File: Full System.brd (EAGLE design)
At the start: 47.5 x 21.5 mm, 46 parts, among them CN2 JSTPH, IC1 MEGA328-A, IC2 L4931D, Q1-M 8MHz, 22pF, U2 MCP73831T-2ACI/OT, U3 FTS31XS-U

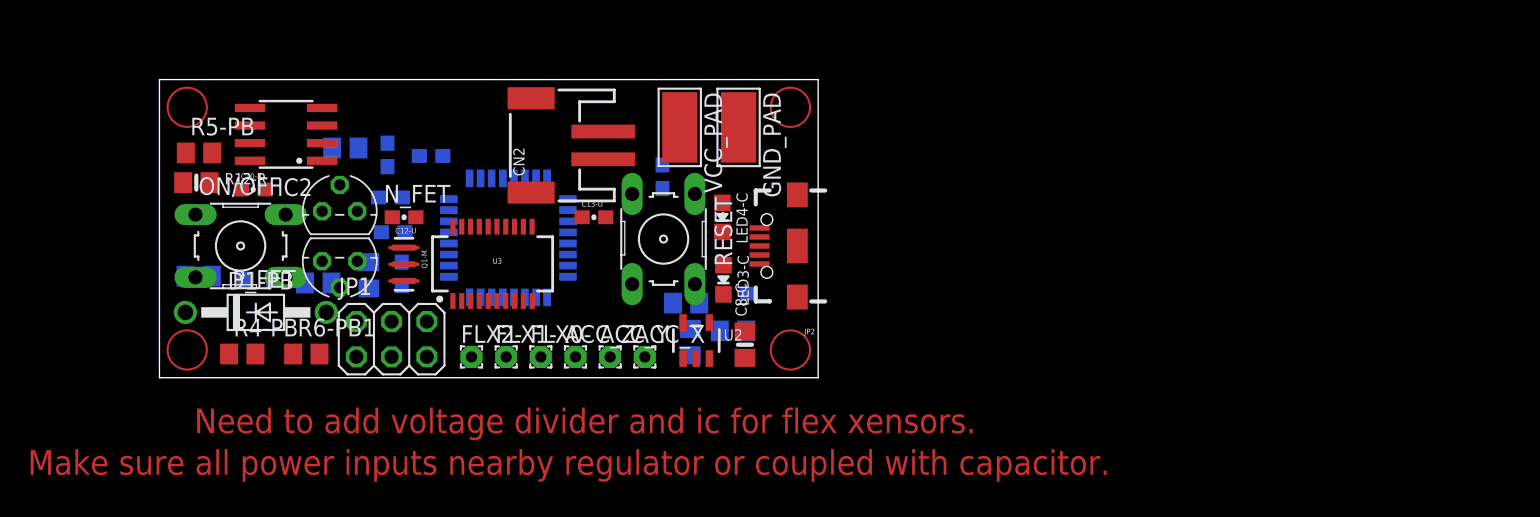
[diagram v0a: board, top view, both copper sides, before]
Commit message: Add files via upload
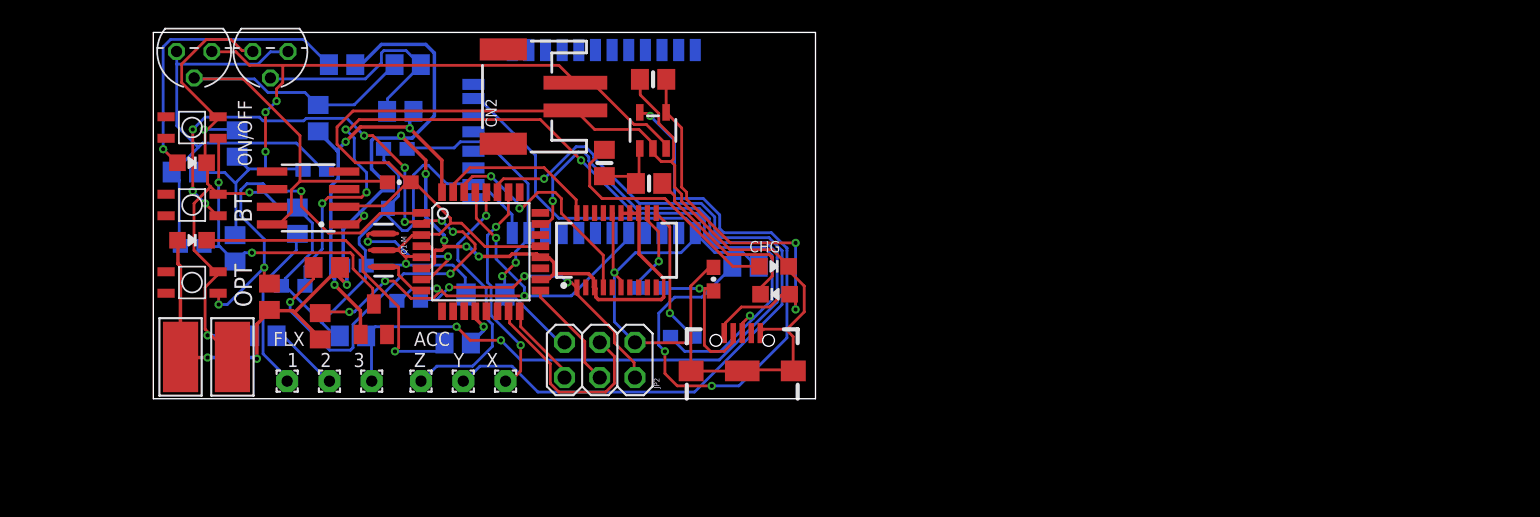
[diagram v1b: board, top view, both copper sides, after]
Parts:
- removed LED4-C: GREEN, microbuilder:CHIPLED_0805_NOOUTLINE
- removed ON/OFF, RESET: (no value), switch-omron:B3F-10XX
- removed R6-PB1: 10k, rcl:R0805
- added C1: 0.1uF, SparkFun:0603-CAP
- added C2: 10uF, SparkFun:EIA3216
- added CHG: GREEN, microbuilder:CHIPLED_0805_NOOUTLINE
- added LED2-M: Blue, microbuilder:CHIPLED_0805_NOOUTLINE
- added R1-M, R1-M1, R1-M2, R1-M3, R2-M, R2-M1, R3-M: 10k, rcl:R0805
- added S1: Power, Spark:TACTILE_SWITCH_SMD
- added S2: Option, Spark:TACTILE_SWITCH_SMD
- added S3: BT_C, Spark:TACTILE_SWITCH_SMD
- added U1: BLUETOOTH-RN41", SparkFun-RF:RN41
- D1-PB: value 1N4004 -> (none); device diode:DO41-10 -> semicon-smd-ipc:SOT23
- moved GND_PAD 40.1 mm to (9.26, 2.00)
- moved VCC_PAD 39.6 mm to (5.52, 2.00), turned to 0 degrees
- moved C14-U 27.5 mm to (18.1, 8.59), turned to 180 degrees
- moved C8-C 20.3 mm to (39.6, 22.0), turned to 180 degrees
- moved R13-U 18.5 mm to (39.5, 6.97)
- moved P_FET 18.4 mm to (6.50, 24.0)
- moved R4-PB 17.9 mm to (15.4, 19.2), flipped to the bottom, turned to 270 degrees
- moved U2 15.5 mm to (39.6, 18.3)
- moved R9-C 15.2 mm to (36.1, 16.0), flipped to the top, turned to 270 degrees
- moved JP1 15.1 mm to (35.7, 1.78)
- moved R5-PB 14.8 mm to (21.4, 19.7), flipped to the bottom, turned to 180 degrees
- moved C7-PB 14.5 mm to (6.36, 10.0)
- moved R12-R 13.5 mm to (17.2, 23.1), flipped to the bottom
- moved C9-C 13.4 mm to (9.60, 17.4), turned to 90 degrees
- moved FLX2- 13.4 mm to (13.2, 0.25)
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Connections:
- removed net N$13: IC1.12
- new net FLX1: FLX1-.1, R1-M2.1
- new net LED1: IC1.12, R2-M1.1
- new net N$10: LED2-M.C, R2-M1.2
- new net N$6: IC1.2, R3-M.1, S3.1
- new net PIO10: U1.33
- new net PIO11: U1.34
- new net PIO2: U1.19
- new net PIO3: U1.20
- new net PIO4: U1.22
- new net PIO5: U1.21
- new net PIO6: U1.3
- new net PIO7: U1.4
- new net RESET: C2-M.1, IC1.29, R1-M.2, U1.5
- new net SPICLK: U1.6
- new net SPICSB: U1.23
- new net SPIMISO: U1.24
- new net SPIMOSI: U1.2
- new net UARTCTS: U1.16
- new net UARTRTS: U1.15
- new net UARTRX: U1.13
- new net UARTTX: U1.14
- net 3.3V: now also LED2-M.A, R1-M.1, R2-M.2, R3-M.2; no longer R6-PB1.1
- net ACC_X: now also ACC_X.1
- net ACC_Y: now also ACC_Y.1
- net ACC_Z: now also ACC_Z.1
- net FLX0: now also FLX0-.1, R1-M1.1
- net GND: now also C1.2, C2.C, CHG.C, R1-M1.2, R1-M2.2, R1-M3.2, S1.2, S2.3, S3.3, U1.1, U1.12, U1.28, U1.29; no longer LED4-C.C, ON/OFF.3, ON/OFF.4, RESET.3, RESET.4
- net N$14: now also FLX2-.1, R1-M3.1; no longer IC1.13
- net N$19: now also CHG.A; no longer LED4-C.A
- net N$2: now also IC1.1, R2-M.1, S2.1; no longer C2-M.1, IC1.29, R6-PB1.2, RESET.1, RESET.2
- net N$5: now also D1-PB.3, S1.4; no longer D1-PB.C, ON/OFF.1, ON/OFF.2
- net POWER_OFF: now also D1-PB.1; no longer D1-PB.A
- net VCC: now also C1.1, C2.A, U1.11
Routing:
- net GND: track 0.00 -> 255.9 mm, vias 0 -> 5
- net 3.3V: track 0.00 -> 101.2 mm, vias 0 -> 9
- net N$12: track 0.00 -> 65.4 mm, vias 0 -> 5
- net FLX0: track 0.00 -> 64.5 mm, vias 0 -> 3
- net VBAT: track 0.00 -> 57.3 mm, vias 0 -> 3
- net N$6: track 0.00 -> 56.9 mm, vias 0 -> 10
- net ACC_Y: track 0.00 -> 56.8 mm, vias 0 -> 1
- net N$18: track 0.00 -> 46.4 mm, vias 0 -> 3
- net V_IN: track 0.00 -> 39.7 mm
- net RESET: track 0.00 -> 38.8 mm, vias 0 -> 5
- net N$15: track 0.00 -> 34.4 mm
- net VBUS: track 0.00 -> 30.9 mm, vias 0 -> 2
- net POWER_OFF: track 0.00 -> 29.2 mm, vias 0 -> 3
- net N$2: track 0.00 -> 28.7 mm, vias 0 -> 3
- net VCC: track 0.00 -> 24.9 mm, vias 0 -> 2
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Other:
- board size 47.5 x 21.5 mm -> 47.8 x 26.4 mm
- board text added: "1 2 3"
- board text added: "ACC"
- board text added: "BT"
- board text added: "FLX"
- board text added: "ON/OFF"
- board text added: "OPT"
- board text added: "Z Y X"
- board text removed: "Make sure all power inputs nearby regulator or coupled with capacitor."
- board text removed: "Need to add voltage divider and ic for flex xensors."
